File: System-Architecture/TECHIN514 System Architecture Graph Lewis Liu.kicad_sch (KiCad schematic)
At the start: 9 parts, among them SW1 SW_Push, SW2 SW_Push, SW3 SW_Push, U1 XIAO ESP32C3, U2 A3144, U3 XIAO ESP32C3

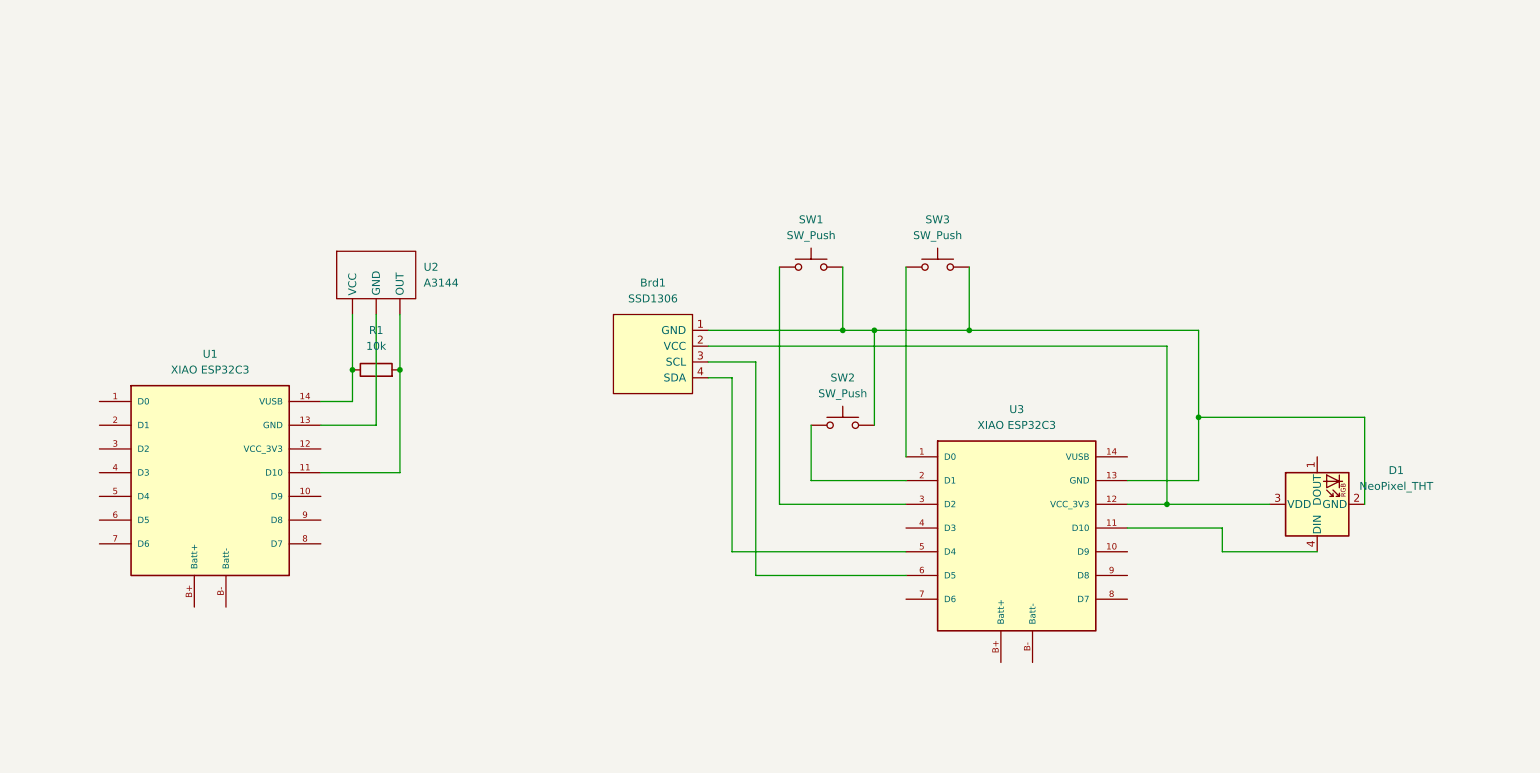
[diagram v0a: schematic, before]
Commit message: update battery life
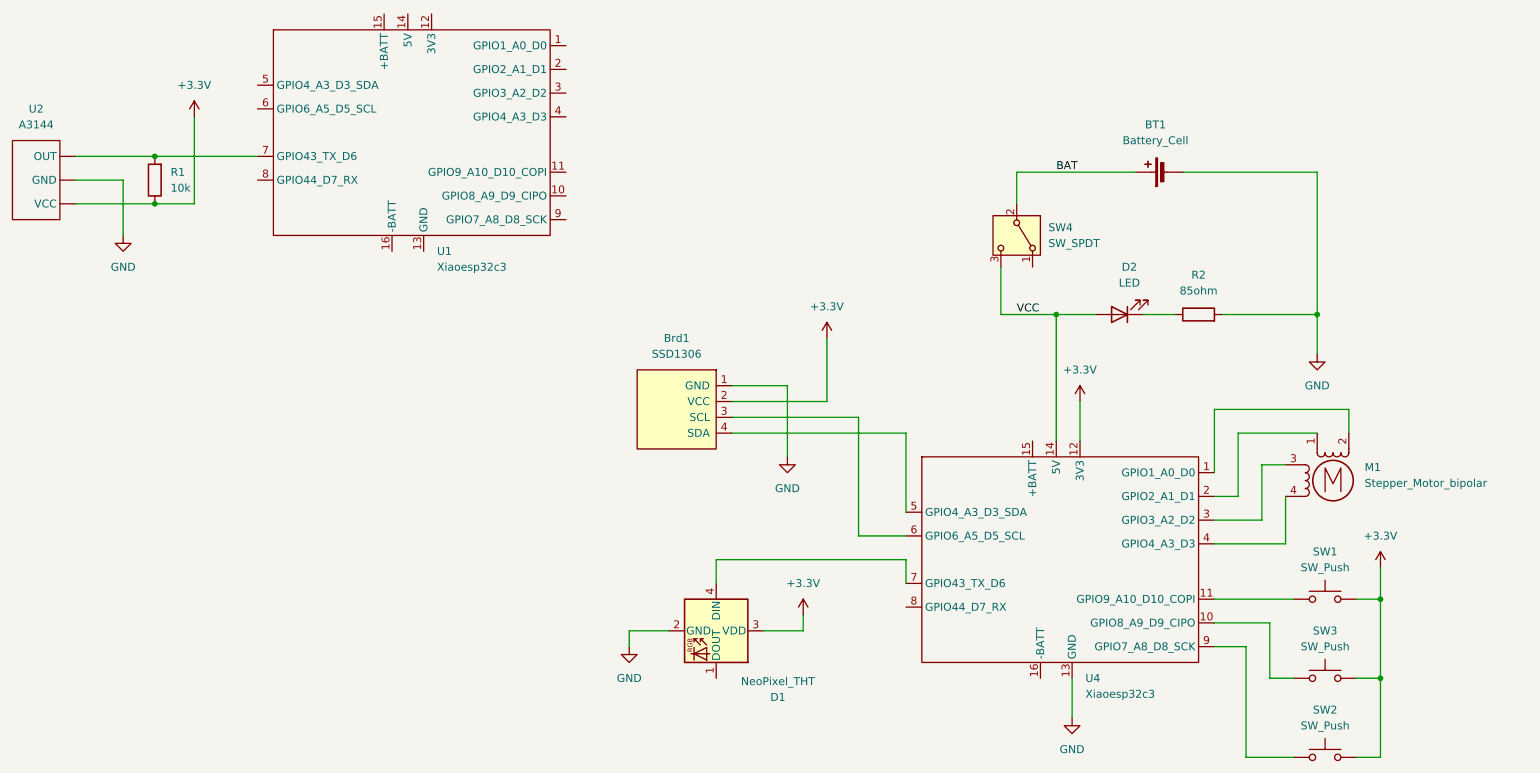
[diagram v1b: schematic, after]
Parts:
- removed U1, U3: XIAO ESP32C3, XIAO_ESP32C3:xiao_esp32c3, symbol xiao_esp32c3:XIAO ESP32C3
- added BT1: Battery_Cell, Connector_PinSocket_2.54mm:PinSocket_1x02_P2.54mm_Vertical, symbol Device:Battery_Cell
- added D2: LED, LED_SMD:LED_0805_2012Metric_Pad1.15x1.40mm_HandSolder, symbol Device:LED
- added M1: Stepper_Motor_bipolar, x27_Footprint:x27_stepper, symbol Motor:Stepper_Motor_bipolar
- added R2: 85ohm, Resistor_SMD:R_0805_2012Metric_Pad1.20x1.40mm_HandSolder, symbol Device:R
- added SW4: SW_SPDT, Connector_PinSocket_2.54mm:PinSocket_1x03_P2.54mm_Vertical, symbol Switch:SW_SPDT
- added U1: Xiaoesp32c3, symbol GIX_ESP32:XIAO_ESP32
- added U4: Xiaoesp32c3, GIX_ESP32:XIAO_ESP32, symbol GIX_ESP32:XIAO_ESP32
- Brd1: footprint (none) -> SSD1306:128x64OLED
- D1: footprint (none) -> Connector_PinSocket_2.54mm:PinSocket_1x04_P2.54mm_Vertical
- SW1, SW2, SW3: footprint (none) -> Connector_PinSocket_2.54mm:PinSocket_1x02_P2.54mm_Vertical
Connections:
- net at SW1.1: now also U4.11 (GPIO9_A10_D10_COPI)
- net +3.3V: now reaches SW1.2, SW2.2, SW3.2
- net +3.3V: now also Brd1.2 (VCC), D1.3 (VDD), R1.1, U2. (OUT), U4.12 (3V3); no longer Brd1.1 (GND), D1.2 (GND)
- net at D1.4 (DIN): now also U4.7 (GPIO43_TX_D6)
- net at SW3.1: now also U4.10 (GPIO8_A9_D9_CIPO)
- net at SW2.1: now also U4.9 (GPIO7_A8_D8_SCK)
- net at Brd1.4 (SDA): now also U4.5 (GPIO4_A3_D3_SDA)
- net at Brd1.3 (SCL): now also U4.6 (GPIO6_A5_D5_SCL)
- net GND: now reaches U2. (OUT)
- net GND: now also Brd1.1 (GND), D1.2 (GND), BT1.2 (-), R2.2, U4.13 (GND); no longer R1.1
- net at R1.2, U2. (OUT): now also U1.7 (GPIO43_TX_D6)
- new net: M1.1, U4.2 (GPIO2_A1_D1)
- new net: M1.2 (-), U4.1 (GPIO1_A0_D0)
- new net: M1.3, U4.3 (GPIO3_A2_D2)
- new net: M1.4, U4.4 (GPIO4_A3_D3)
- new net: D2.1 (K), R2.1
- new net BAT: BT1.1 (+), SW4.2 (B)
- new net VCC: D2.2 (A), SW4.3 (C), U4.14 (5V)
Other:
- company: (none) -> Lewis Liu
- moved on the sheet: Brd1, D1, R1, SW1, SW2, SW3, U2
